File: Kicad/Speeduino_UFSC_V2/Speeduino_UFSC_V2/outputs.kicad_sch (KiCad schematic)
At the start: 16 parts, among them J3 Conn_01x06, Q2 Q_NMOS_GDSD, Q3 HVM NMOS, U5 ULN2003

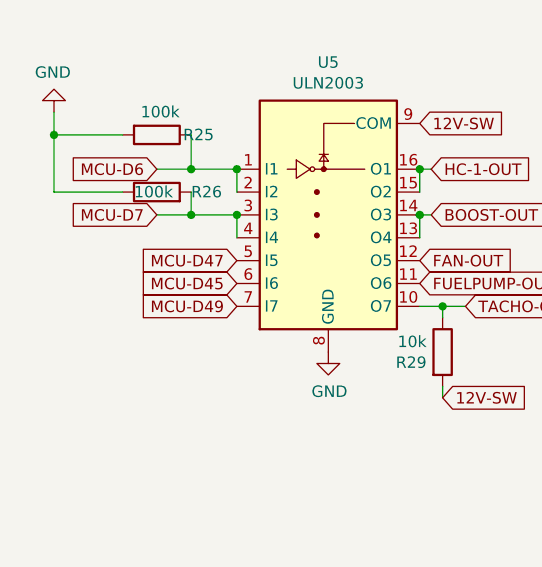
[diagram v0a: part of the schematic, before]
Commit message: Add pdf
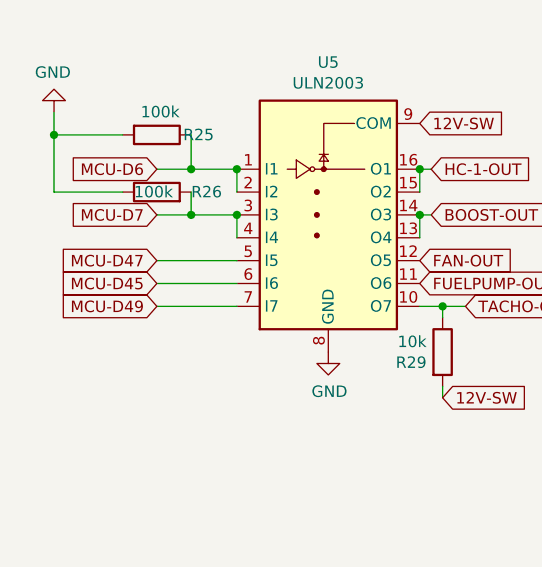
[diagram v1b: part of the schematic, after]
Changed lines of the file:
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@@
 	(wire
 		(pts
+			(xy 57.15 73.66) (xy 66.04 73.66)
+		)
+		(stroke
+			(width 0)
+			(type default)
+		)
+	)
+	(wire
+		(pts
 			(xy 189.23 48.26) (xy 196.85 48.26)
 		)
@@
 	(wire
 		(pts
+			(xy 57.15 71.12) (xy 66.04 71.12)
+		)
+		(stroke
+			(width 0)
+			(type default)
+		)
+	)
+	(wire
+		(pts
 			(xy 214.63 33.02) (xy 223.52 33.02)
 		)
@@
 	(wire
 		(pts
+			(xy 57.15 68.58) (xy 66.04 68.58)
+		)
+		(stroke
+			(width 0)
+			(type default)
+		)
+	)
+	(wire
+		(pts
 			(xy 196.85 48.26) (xy 196.85 46.99)
 		)
@@
 	(global_label "MCU-D49"
 		(shape input)
-		(at 66.04 73.66 180)
+		(at 57.15 73.66 180)
 		(effects
 			(font
@@
 		)
 		(property "Intersheetrefs" "${INTERSHEET_REFS}"
-			(at 66.04 73.66 0)
+			(at 57.15 73.66 0)
 			(effects
 				(font
@@
 	(global_label "MCU-D45"
 		(shape input)
-		(at 66.04 71.12 180)
+		(at 57.15 71.12 180)
 		(effects
 			(font
@@
 		)
 		(property "Intersheetrefs" "${INTERSHEET_REFS}"
-			(at 66.04 71.12 0)
+			(at 57.15 71.12 0)
 			(effects
 				(font
@@
 	(global_label "MCU-D47"
 		(shape input)
-		(at 66.04 68.58 180)
+		(at 57.15 68.58 180)
 		(effects
 			(font
@@
 		)
 		(property "Intersheetrefs" "${INTERSHEET_REFS}"
-			(at 66.04 68.58 0)
+			(at 57.15 68.58 0)
 			(effects
 				(font
@@
 			)
 		)
-		(property "Description" ""
+		(property "Description" "Resistor"
 			(at 64.77 144.78 0)
 			(effects
@@
 			)
 		)
-		(property "Description" ""
+		(property "Description" "Power symbol creates a global label with name \"GND\" , ground"
 			(at 214.63 46.99 0)
 			(effects
@@
 			)
 		)
-		(property "Description" ""
+		(property "Description" "N-MOSFET transistor, drain/gate/source"
 			(at 212.09 63.5 0)
 			(effects
@@
 			)
 		)
-		(property "Description" ""
+		(property "Description" "Resistor"
 			(at 207.01 68.58 0)
 			(effects
@@
 			)
 		)
-		(property "Description" ""
+		(property "Description" "Diode"
 			(at 227.33 38.1 0)
 			(effects
@@
 			)
 		)
+		(property "Sim.Device" "D"
+			(at 227.33 38.1 0)
+			(effects
+				(font
+					(size 1.27 1.27)
+				)
+				(hide yes)
+			)
+		)
+		(property "Sim.Pins" "1=K 2=A"
+			(at 227.33 38.1 0)
+			(effects
+				(font
+					(size 1.27 1.27)
+				)
+				(hide yes)
+			)
+		)
 		(pin "1"
 		)
@@
 			)
 		)
-		(property "Description" ""
+		(property "Description" "High Voltage, High Current Darlington Transistor Arrays, SOIC16/SOIC16W/DIP16/TSSOP16"
 			(at 76.2 63.5 0)
 			(effects
@@
 			)
 		)
-		(property "Description" ""
+		(property "Description" "Resistor"
 			(at 88.9 78.74 0)
 			(effects
@@
 			)
 		)
-		(property "Description" ""
+		(property "Description" "Power symbol creates a global label with name \"GND\" , ground"
 			(at 66.04 156.21 0)
 			(effects
@@
 			)
 		)
-		(property "Description" ""
+		(property "Description" "Power symbol creates a global label with name \"GND\" , ground"
 			(at 227.33 149.86 0)
 			(effects
@@
 			)
 		)
-		(property "Description" ""
+		(property "Description" "Resistor"
 			(at 196.85 68.58 0)
 			(effects
@@
 			)
 		)
-		(property "Description" ""
+		(property "Description" "Power symbol creates a global label with name \"GND\" , ground"
 			(at 45.72 52.07 0)
 			(effects
@@
 			)
 		)
-		(property "Description" ""
+		(property "Description" "Resistor"
 			(at 196.85 43.18 0)
 			(effects
@@
 			)
 		)
-		(property "Description" ""
+		(property "Description" "Resistor"
 			(at 207.01 43.18 0)
 			(effects
@@
 			)
 		)
-		(property "Description" ""
+		(property "Description" "Diode"
 			(at 227.33 63.5 0)
 			(effects
@@
 			)
 		)
+		(property "Sim.Device" "D"
+			(at 227.33 63.5 0)
+			(effects
+				(font
+					(size 1.27 1.27)
+				)
+				(hide yes)
+			)
+		)
+		(property "Sim.Pins" "1=K 2=A"
+			(at 227.33 63.5 0)
+			(effects
+				(font
+					(size 1.27 1.27)
+				)
+				(hide yes)
+			)
+		)
 		(pin "1"
 		)
@@
 			)
 		)
-		(property "Description" ""
+		(property "Description" "Power symbol creates a global label with name \"GND\" , ground"
 			(at 196.85 63.5 0)
 			(effects
@@
 			)
 		)
-		(property "Description" ""
+		(property "Description" "Resistor"
 			(at 57.15 54.61 0)
 			(effects
@@
 			)
 		)
-		(property "Description" ""
+		(property "Description" "Power symbol creates a global label with name \"GND\" , ground"
 			(at 214.63 72.39 0)
 			(effects
@@
 			)
 		)
-		(property "Description" ""
+		(property "Description" "Pololu Breakout Board, Stepper Driver DRV8825"
 			(at 219.71 127 0)
 			(effects
@@
 			)
 		)
-		(property "Description" ""
+		(property "Description" "Resistor"
 			(at 71.12 151.13 0)
 			(effects
@@
 			)
 		)
-		(property "Description" ""
+		(property "Description" "Power symbol creates a global label with name \"GND\" , ground"
 			(at 64.77 138.43 0)
 			(effects
@@
 			)
 		)
-		(property "Description" ""
+		(property "Description" "Resistor"
 			(at 57.15 60.96 0)
 			(effects
@@
 			)
 		)
-		(property "Description" ""
+		(property "Description" "N-MOSFET transistor, drain/gate/source"
 			(at 212.09 38.1 0)
 			(effects
@@
 			)
 		)
-		(property "Description" ""
+		(property "Description" "Power symbol creates a global label with name \"GND\" , ground"
 			(at 196.85 38.1 0)
 			(effects
@@
 			)
 		)
-		(property "Description" ""
+		(property "Description" "Generic connector, single row, 01x06, script generated (kicad-library-utils/schlib/autogen/connector/)"
 			(at 55.88 156.21 0)
 			(effects
@@
 			)
 		)
-		(property "Description" ""
+		(property "Description" "Power symbol creates a global label with name \"GND\" , ground"
 			(at 76.2 78.74 0)
 			(effects
